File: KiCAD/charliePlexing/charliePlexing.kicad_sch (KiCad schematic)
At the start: 0 parts

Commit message: First build
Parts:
- added C1: 100nF, symbol Device:C
- added D1, D10, D11, D12, D2, D3, D4, D5, D6, D7, D8, D9: LED, symbol Device:LED
- added SW1: mode, symbol Switch:SW_MEC_5G
- added U2: ~, symbol stm8l050j3:STM8L001J3
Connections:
- new net: SW1.3 (B), SW1.4 (B), U2.2 (PA2)
- new net 3.3Vdd: C1.1, U2.4 (VDD)
- new net GND: C1.2, SW1.1 (A), SW1.2 (A), U2.3 (VSS)
- new net PB5: D10.2 (A), D11.2 (A), D12.2 (A), D3.1 (K), D6.1 (K), D9.1 (K), U2.5 (PB3/5)
- new net PB6: D12.1 (K), D2.1 (K), D5.1 (K), D7.2 (A), D8.2 (A), D9.2 (A), U2.6 (PB6)
- new net PB7: D1.1 (K), D11.1 (K), D4.2 (A), D5.2 (A), D6.2 (A), D8.1 (K), U2.7 (I2C_SDA)
- new net PC1: D1.2 (A), D10.1 (K), D2.2 (A), D3.2 (A), D4.1 (K), D7.1 (K), U2.8 (I2C_SCL)
- new net programming: U2.1 (SWIM)
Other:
- note added: "CharliePlexing demo"

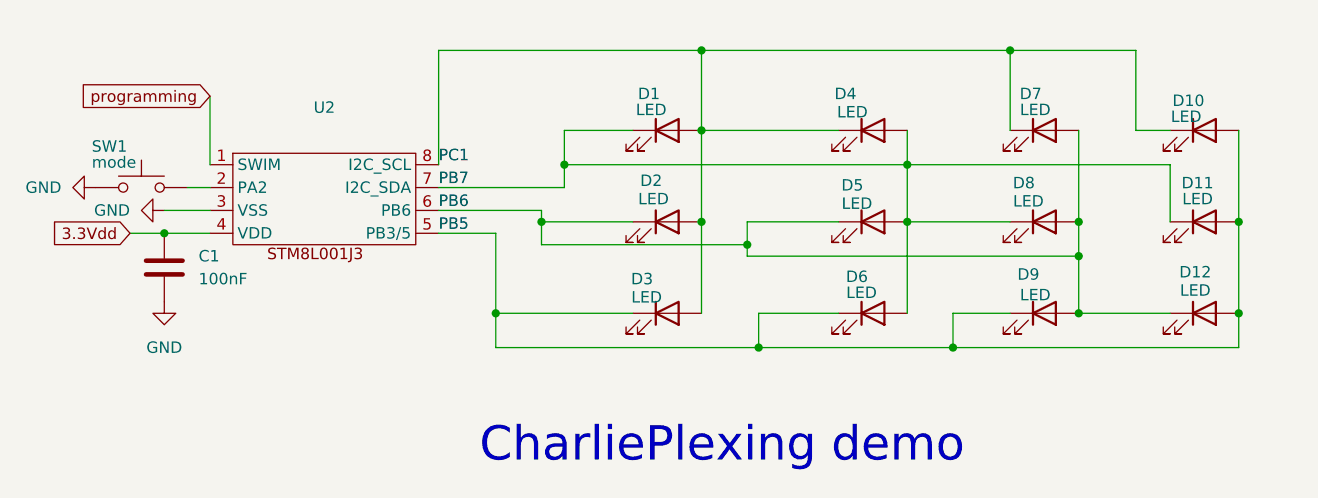
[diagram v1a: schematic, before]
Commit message: premier test du démo
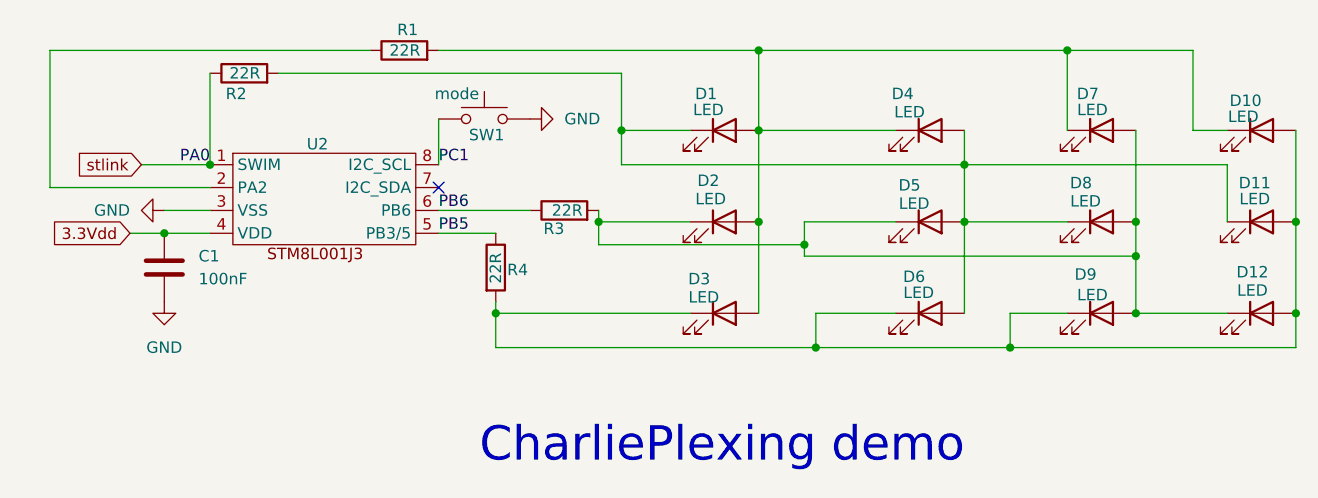
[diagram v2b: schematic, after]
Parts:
- added R1, R2, R3, R4: 22R, symbol Device:R
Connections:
- net GND: now also SW1.3 (B), SW1.4 (B); no longer SW1.1 (A), SW1.2 (A)
- net PB5: now also R4.1; no longer D10.2 (A), D11.2 (A), D12.2 (A), D3.1 (K), D6.1 (K), D9.1 (K)
- net PB6: now also R3.1; no longer D12.1 (K), D2.1 (K), D5.1 (K), D7.2 (A), D8.2 (A), D9.2 (A)
- net PC1: now also SW1.1 (A), SW1.2 (A); no longer D1.2 (A), D10.1 (K), D2.2 (A), D3.2 (A), D4.1 (K), D7.1 (K)
- net PB7: no longer names the net of D1.1 (K), D11.1 (K), D4.2 (A), D5.2 (A), D6.2 (A), D8.1 (K)
- net PB7: now also R2.2; no longer U2.7 (I2C_SDA)
- net programming renamed stlink
- net stlink: now also R2.1
- new net: D12.1 (K), D2.1 (K), D5.1 (K), D7.2 (A), D8.2 (A), D9.2 (A), R3.2
- new net: D1.2 (A), D10.1 (K), D2.2 (A), D3.2 (A), D4.1 (K), D7.1 (K), R1.2
- new net: R1.1, U2.2 (PA2)
- new net: D10.2 (A), D11.2 (A), D12.2 (A), D3.1 (K), D6.1 (K), D9.1 (K), R4.2
- no-connect marks 0 -> 1
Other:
- moved on the sheet: D1, D10, D11, D12, D2, D3, D4, D5, D6, D7, D8, D9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
